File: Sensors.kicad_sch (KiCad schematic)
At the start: 6 parts, among them U2 SHT31-ARP-B

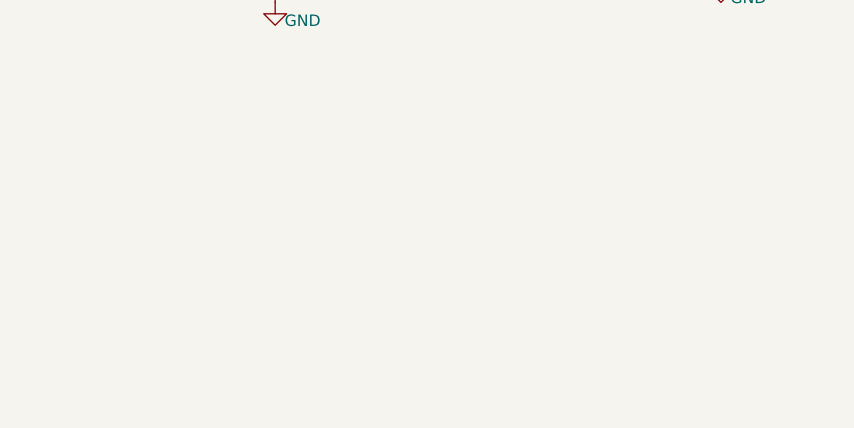
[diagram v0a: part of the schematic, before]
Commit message: Add files via upload
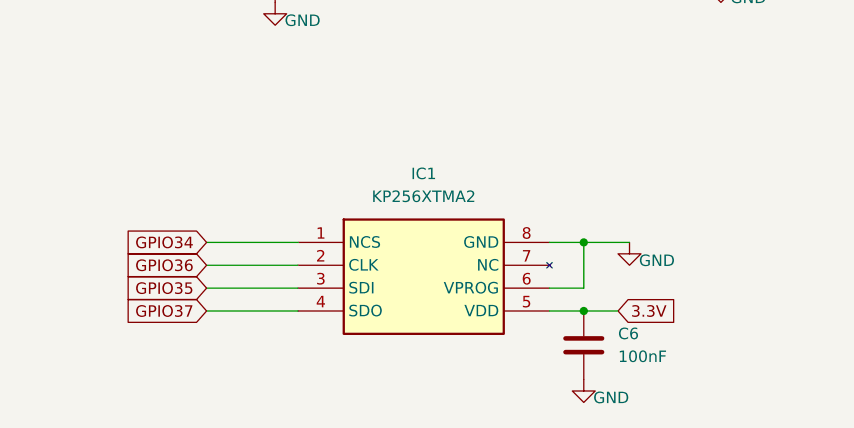
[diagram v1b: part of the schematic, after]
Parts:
- added C6: 100nF, Capacitor_SMD:C_0805_2012Metric_Pad1.18x1.45mm_HandSolder, symbol Device:C
- added IC1: KP256XTMA2, Weather Station:KP256XTMA2, symbol pressuresens:KP256XTMA2
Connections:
- net 3.3V: now also C6.1, IC1.5 (VDD)
- net GND: now also C6.2, IC1.6 (VPROG), IC1.8 (GND)
- new net GPIO34: IC1.1 (NCS)
- new net GPIO35: IC1.3 (SDI)
- new net GPIO36: IC1.2 (CLK)
- new net GPIO37: IC1.4 (SDO)
